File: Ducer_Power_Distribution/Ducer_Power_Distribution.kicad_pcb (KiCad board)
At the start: 2 copper layers, 115 x 67 mm, 17 parts, among them J1 Mini_Fit_Jr_1x3_pin, J10 Conn_01x05, J11 Power In, J2 Mini_Fit_Jr_1x3_pin, J3 Mini_Fit_Jr_1x3_pin, J4 Mini_Fit_Jr_1x3_pin, J5 Mini_Fit_Jr_1x3_pin, J6 Mini_Fit_Jr_1x3_pin, J7 Mini_Fit_Jr_1x3_pin, J8 Mini_Fit_Jr_1x3_pin, J9 Conn_01x05

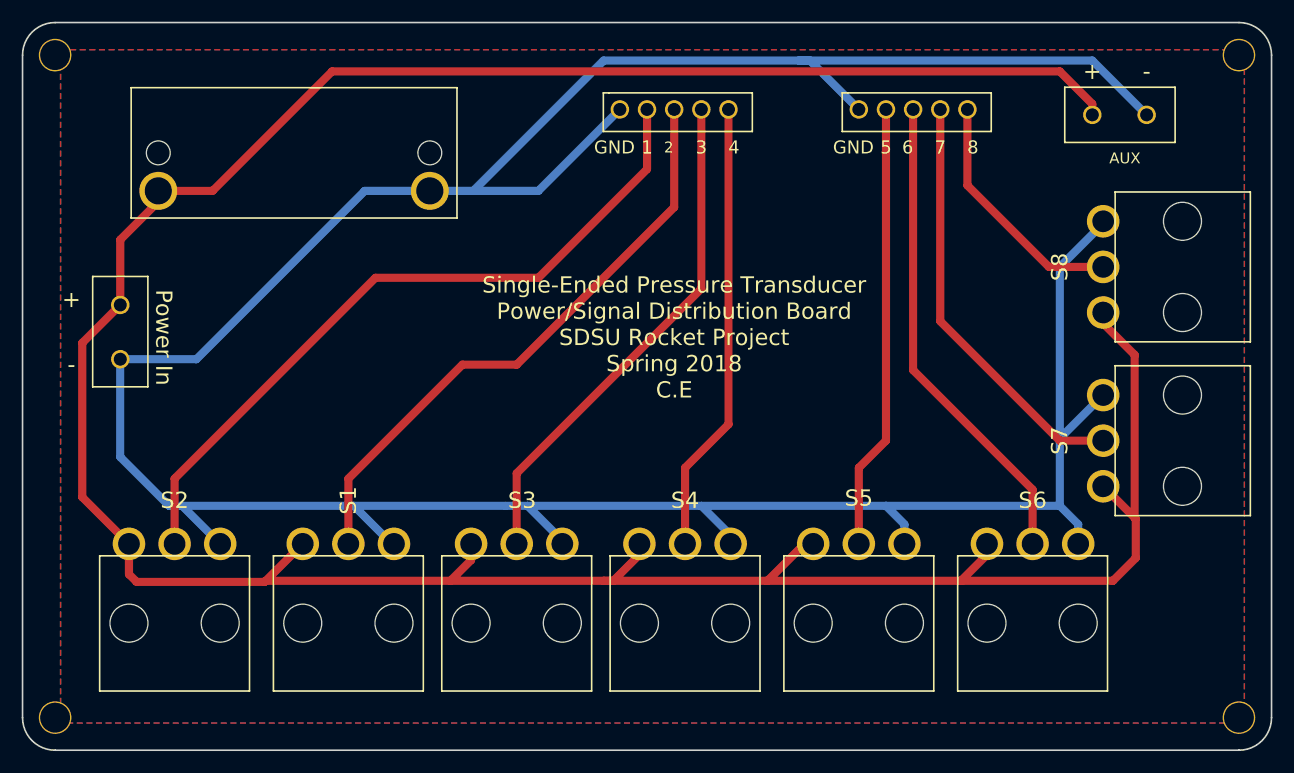
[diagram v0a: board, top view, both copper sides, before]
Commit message: pre-purging AvTop
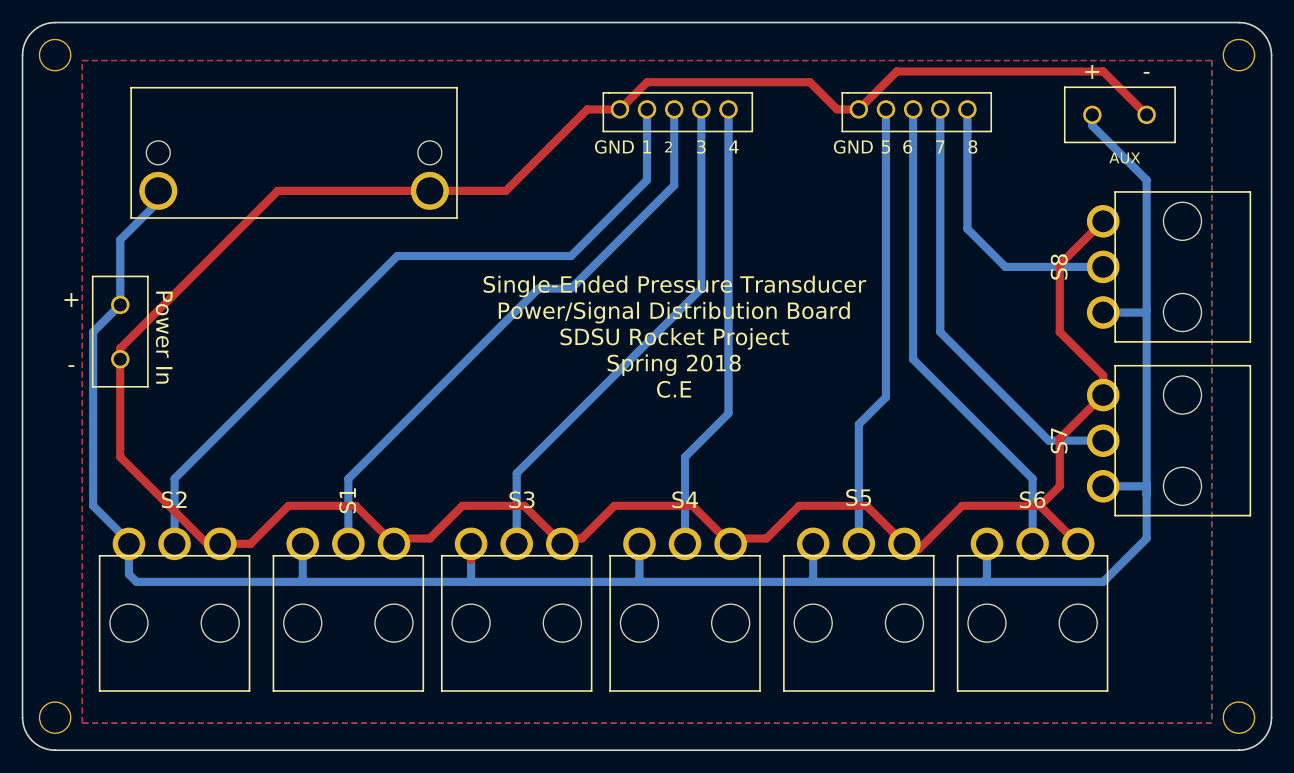
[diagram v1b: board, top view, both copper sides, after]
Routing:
- net VCC: track 286.0 -> 219.1 mm
- net GND: track 291.2 -> 257.7 mm
- net Net-(J10-Pad5): track 24.8 -> 27.1 mm
- net Net-(J2-Pad2): track 56.4 -> 55.2 mm
- net Net-(J10-Pad4): track 40.5 -> 41.0 mm
- net Net-(J1-Pad2): track 66.8 -> 67.4 mm
